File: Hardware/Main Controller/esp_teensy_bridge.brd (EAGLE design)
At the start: 102.8 x 87.9 mm, 47 parts, among them IC1 BQ79600PWRQ1, Q1 SI7611DN-T1-GE3, Q2 SI7611DN-T1-GE3, Q3 SI7611DN-T1-GE3, Q4 SI7611DN-T1-GE3

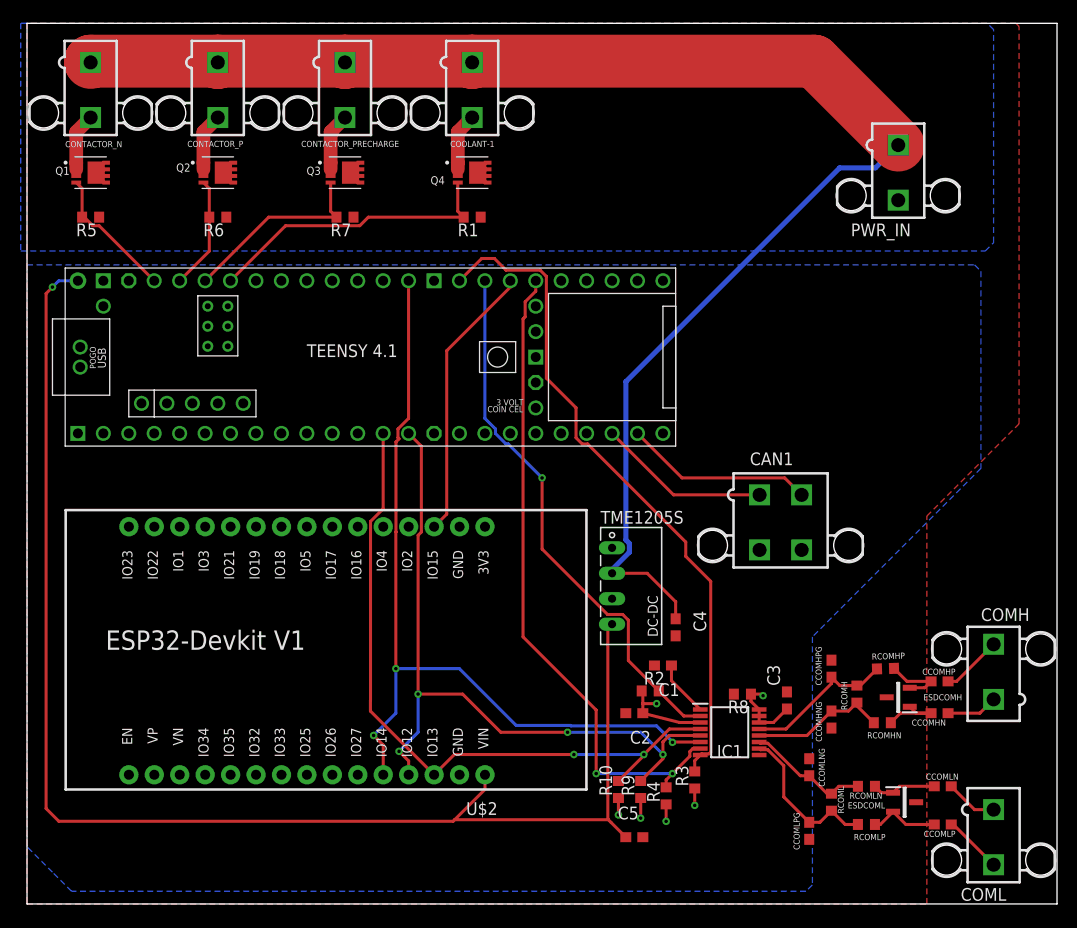
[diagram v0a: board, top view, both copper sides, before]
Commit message: design review changes
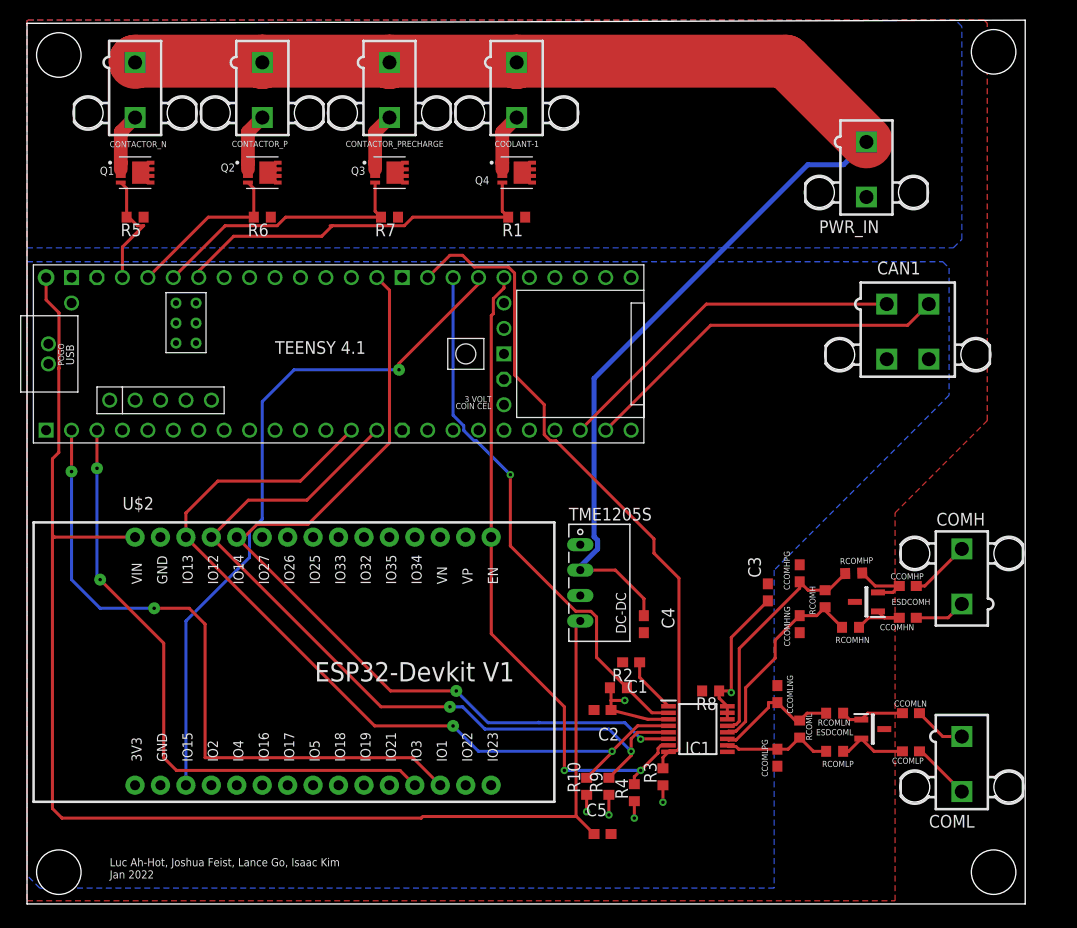
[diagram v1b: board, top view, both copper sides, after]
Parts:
- moved CAN1 22.9 mm to (87.9, 57.1)
- moved C3 11.0 mm to (74.0, 31.1)
- moved U$2 10.9 mm to (33.7, 25.4), turned to 0 degrees
- moved ESDCOMH 10.0 mm to (83.8, 30.2)
- moved RCOMH 10.0 mm to (79.7, 30.5)
- moved CCOMHNG 10.0 mm to (77.2, 27.9)
- moved CCOMHPG 10.0 mm to (77.2, 33.0)
- moved COMH 10.0 mm to (93.3, 32.7)
- moved RCOMHP 10.0 mm to (82.5, 33.0)
- moved CCOMHN 10.0 mm to (87.9, 28.6)
- moved CCOMHP 10.0 mm to (87.9, 31.8)
- moved RCOMHN 10.0 mm to (82.2, 27.6)
- moved CCOMLN 7.96 mm to (88.3, 19.1)
- moved CCOMLP 7.96 mm to (88.3, 15.2)
- moved CCOMLPG 7.96 mm to (74.9, 14.6)
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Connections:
- net RX_ESP: now also U$2.12
- net TX_ESP: now also U$2.13
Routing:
- net TX_ESP: track 0.00 -> 68.1 mm, vias 0 -> 2
- net RX_ESP: track 0.00 -> 61.7 mm, vias 0 -> 2
- net CS1: track 27.7 -> 68.9 mm, vias 0 -> 1
- net N$8: track 18.9 -> 37.5 mm
- net N$7: track 17.3 -> 35.8 mm
- net MOSI: track 69.4 -> 84.2 mm
- net MISO: track 71.7 -> 80.5 mm, vias 4 -> 2
- net COOLANT_CTRL: track 29.6 -> 37.7 mm
- net COMHP: track 15.3 -> 23.4 mm
- net VCC: track 150.8 -> 143.0 mm
- net CONTACTORPRECHARGE_CTRL: track 19.4 -> 26.9 mm
- net COMHN: track 13.8 -> 20.7 mm
- net CONTACTORP_CTRL: track 11.3 -> 16.8 mm
- net COMLP: track 15.8 -> 11.1 mm
- net 5V: track 164.2 -> 168.8 mm, vias 7 -> 6
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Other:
- board size 102.8 x 87.9 mm -> 99.7 x 88.3 mm
- board text added: "BMS Main Board V1"
- board text added: "Luc Ah-Hot, Joshua Feist, Lance Go, Isaac Kim Jan 2022"
